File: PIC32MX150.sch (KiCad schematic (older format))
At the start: 28 parts, among them J1 GPIO_1, J2 USB_B_Micro, J3 Barrel_Jack, J4 ICSP, J5 GPIO_2, SW1 RST, SW2 SW_SPDT, U1 PIC32MX150F128D-IPT, U2 LM22676MR-ADJ, U3 CH340C

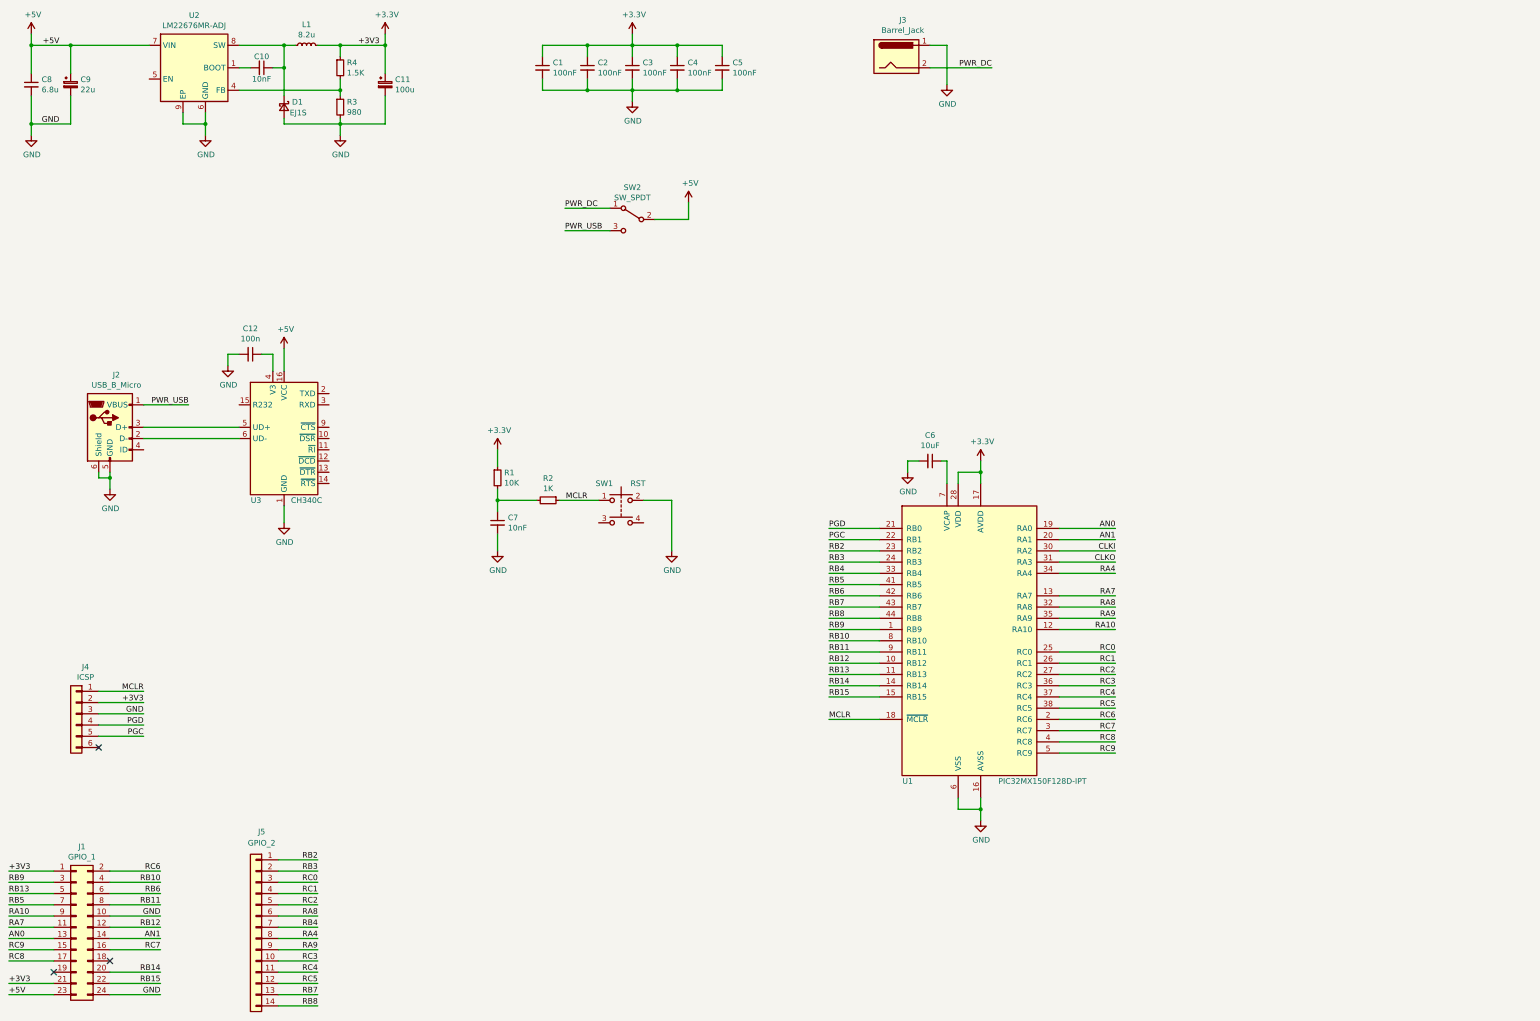
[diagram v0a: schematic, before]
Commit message: LO
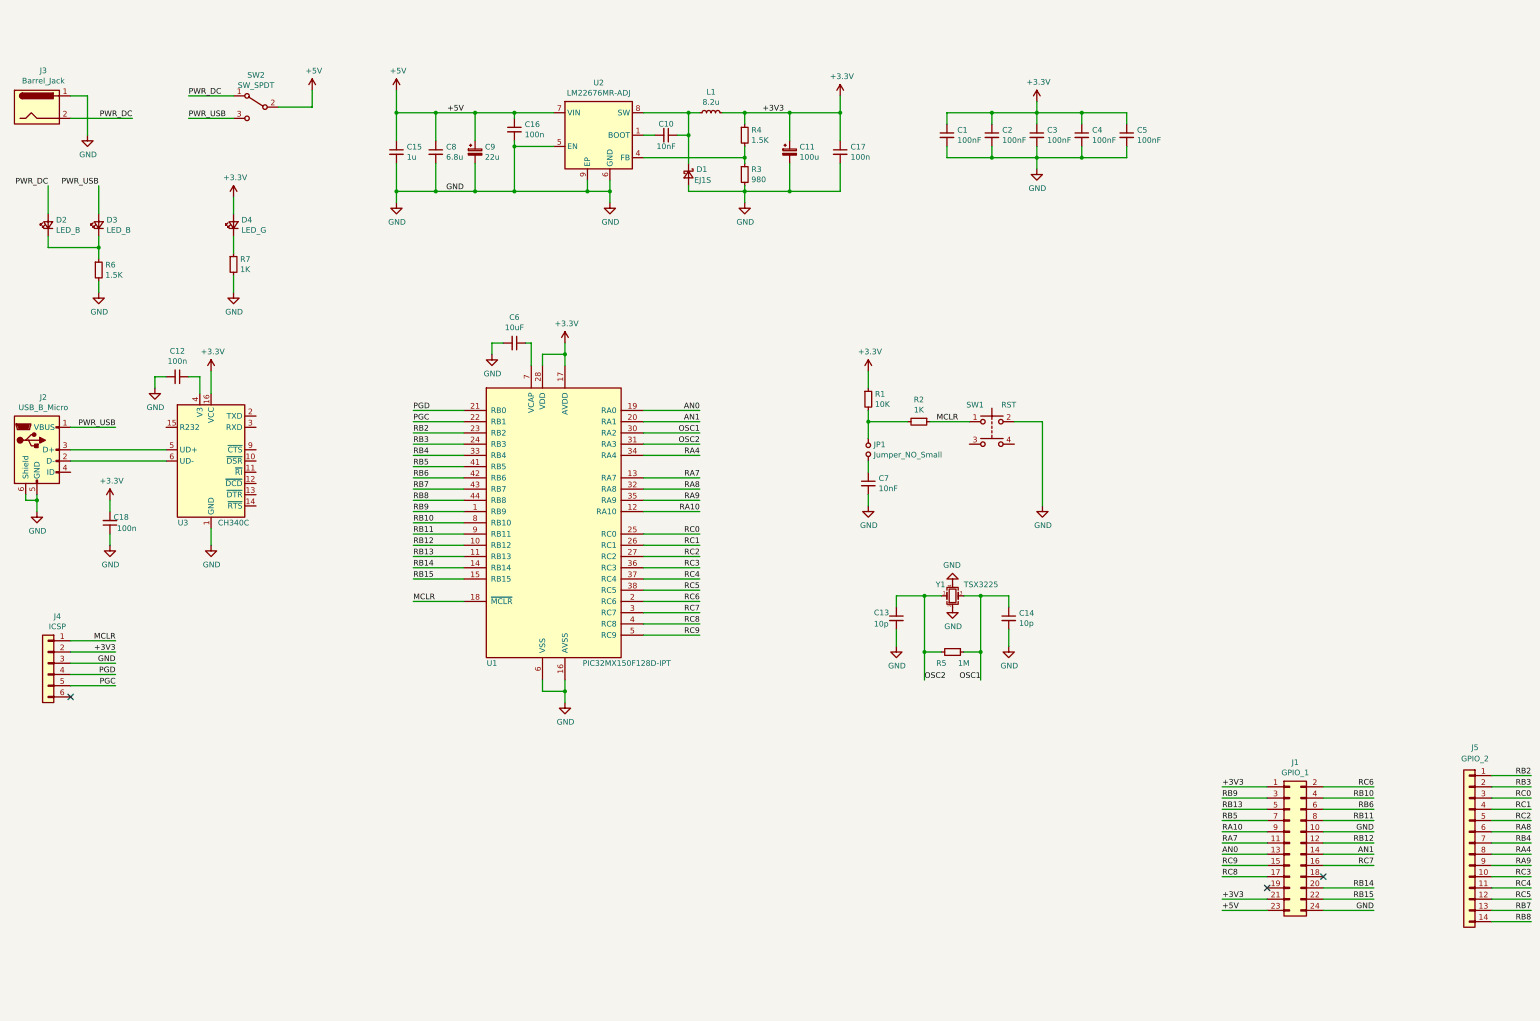
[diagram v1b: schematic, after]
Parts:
- added C13, C14: 10p, Capacitor_SMD:C_0603_1608Metric_Pad1.08x0.95mm_HandSolder, symbol Device:C_Small
- added C15: 1u, Capacitor_SMD:C_0603_1608Metric_Pad1.08x0.95mm_HandSolder, symbol Device:C_Small
- added C16, C17, C18: 100n, Capacitor_SMD:C_0603_1608Metric_Pad1.08x0.95mm_HandSolder, symbol Device:C_Small
- added D2, D3: LED_B, LED_SMD:LED_0603_1608Metric_Pad1.05x0.95mm_HandSolder, symbol Device:LED_Small
- added D4: LED_G, LED_SMD:LED_0603_1608Metric_Pad1.05x0.95mm_HandSolder, symbol Device:LED_Small
- added JP1: Jumper_NO_Small, Jumper:SolderJumper-2_P1.3mm_Open_Pad1.0x1.5mm, symbol Device:Jumper_NO_Small
- added R5: 1M, Resistor_SMD:R_0603_1608Metric_Pad0.98x0.95mm_HandSolder, symbol Device:R_Small
- added R6: 1.5K, Resistor_SMD:R_0603_1608Metric_Pad0.98x0.95mm_HandSolder, symbol Device:R_Small
- added R7: 1K, Resistor_SMD:R_0603_1608Metric_Pad0.98x0.95mm_HandSolder, symbol Device:R_Small
- added Y1: TSX3225, Crystal:Crystal_SMD_SeikoEpson_TSX3225-4Pin_3.2x2.5mm_HandSoldering, symbol Device:Crystal_GND24_Small
- J1: footprint Connector_PinHeader_2.54mm:PinHeader_2x12_P2.54mm_Vertical -> Connector_PinSocket_2.54mm:PinSocket_2x12_P2.54mm_Vertical
- L1: footprint Inductor_SMD:L_0805_2012Metric_Pad1.15x1.40mm_HandSolder -> Inductor_SMD:L_Taiyo-Yuden_MD-1616
- SW2: footprint Button_Switch_THT:SW_Slide_1P2T_CK_OS102011MS2Q -> Custom_Libs:SPDT_SW_Big
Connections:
- net +3V3: now also U3.16 (VCC), C17.1, C18.2, D4.2 (A)
- net +5V: now also C15.1, C16.1; no longer U3.16 (VCC)
- net GND: now also U2.5 (EN), C13.2, C14.2, C15.2, C16.2, C17.2, C18.1, R6.2, R7.2, Y1.2, Y1.4
- net PWR_DC: now also D2.2 (A)
- net PWR_USB: now also D3.2 (A)
- net at R1.2, R2.2: now also JP1.1; no longer C7.1
- net CLKI renamed OSC1
- net OSC1: now also C14.1, R5.1, Y1.3
- net CLKO renamed OSC2
- net OSC2: now also C13.1, R5.2, Y1.1
- new net: C7.1, JP1.2
- new net: D4.1 (K), R7.1
- new net: D2.1 (K), D3.1 (K), R6.1
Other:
- moved on the sheet: C1, C10, C11, C12, C2, C3, C4, C5, C6, C7, C8, C9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
